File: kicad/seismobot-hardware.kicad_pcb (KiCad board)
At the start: 4 copper layers, 80 x 120 mm, 100 parts, among them J1 Screw_Terminal_01x02, J2 Raspberry_Pi_2_3, U1 OPA2156xD, U10 AP7340, U2 OPA2156xD, U3 ref-6, U4 ref-8, U5 LTC6011, U6 OPA2156xD, U7 OPA2156xD, U8 MAX11200, U9 ATSAMD09C13A-SS, X1 SG-5032CAN, Y1 Crystal

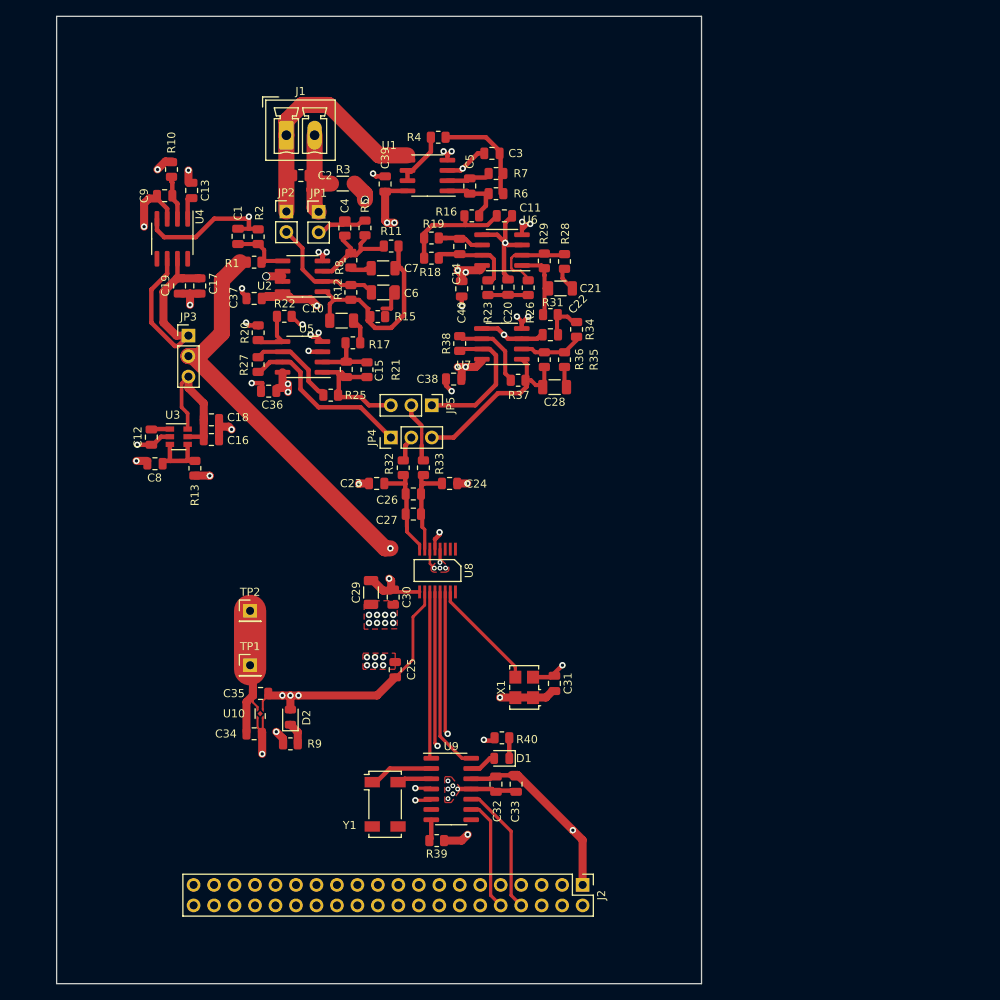
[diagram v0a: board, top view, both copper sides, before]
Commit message: finishing touches before sending out rev 1
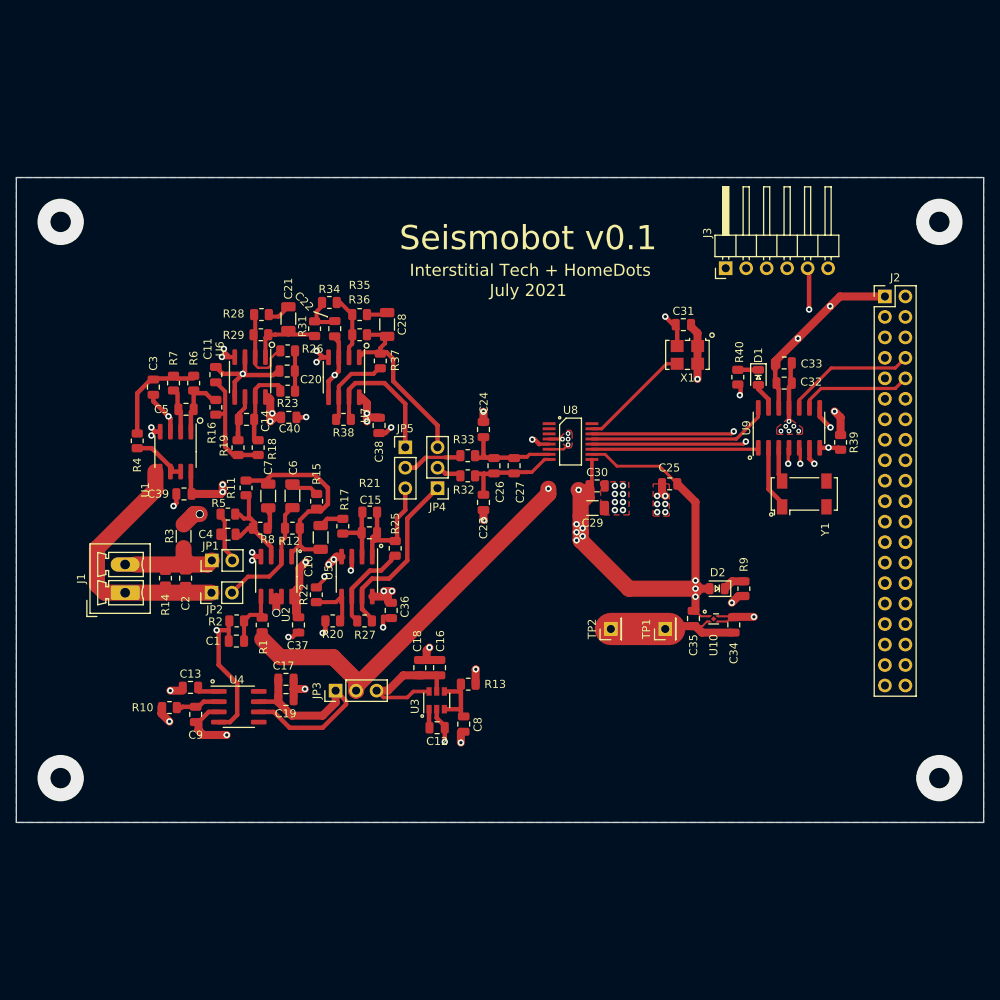
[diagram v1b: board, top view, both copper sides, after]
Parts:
- added J3: Conn_01x06_Male, Connector_PinHeader_2.54mm:PinHeader_1x06_P2.54mm_Horizontal, F.Cu at (183.0, 81.2)
- added R14: DNP, Resistor_SMD:R_0805_2012Metric, F.Cu at (113.5, 119.7)
- moved J2 82.1 mm to (202.8, 84.8), turned to 0 degrees
- moved R39 70.4 mm to (197.2, 102.8), turned to 270 degrees
- moved R10 66.8 mm to (114.0, 135.8), turned to 0 degrees
- moved Y1 64.7 mm to (192.8, 109.2), turned to 90 degrees
- moved C9 64.5 mm to (117.2, 136.6), turned to 90 degrees
- moved C33 61.9 mm to (190.2, 93.0), turned to 0 degrees
- moved C13 61.7 mm to (116.6, 133.2), turned to 0 degrees
- moved U9 61.3 mm to (190.8, 101.0), turned to 90 degrees
- moved C32 61.3 mm to (190.2, 95.5), turned to 180 degrees
- moved C34 61.0 mm to (184.0, 125.5), turned to 270 degrees
- moved J1 60.2 mm to (108.5, 121.5), turned to 90 degrees
- moved R9 59.5 mm to (185.2, 121.0), turned to 90 degrees
- moved U4 58.6 mm to (122.6, 135.7), turned to 0 degrees
- moved U10 57.5 mm to (181.5, 124.8), turned to 0 degrees
- moved D1 57.0 mm to (187.1, 94.8), turned to 270 degrees
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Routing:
- net SWCLK: track 2.69 -> 31.5 mm, vias 0 -> 1
- net ~RST: track 0.00 -> 26.8 mm, vias 0 -> 2
- net SWDIO: track 0.00 -> 25.0 mm, vias 0 -> 1
- net +3V3: track 112.5 -> 135.8 mm, vias 16 -> 21
- net VDD: track 39.5 -> 54.1 mm, vias 2 -> 3
- net G-: track 29.7 -> 31.6 mm
- net GND: track 103.4 -> 103.9 mm
- net (no net): vias 0 -> 4
- added copper zone on B.Cu, net (none)
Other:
- board size 80 x 120 mm -> 120 x 80 mm
- board text added: "Interstitial Tech + HomeDots"
- board text added: "July 2021"
- board text added: "Seismobot v0.1"
- board text added: "These additions were written by resident shepherds and guardians of the Bay Area Makerfarm:"
- board text added: "[thank you, marie]"
